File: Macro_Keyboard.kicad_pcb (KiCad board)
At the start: 6 copper layers, 109.7 x 84.3 mm, 106 parts, among them J1 USB_C_Receptacle_USB2.0, J2 USB_A, J3 USB_A, J4 USB_A, SW1 SW_Push, SW10 SW_DIP_x01, SW2 SW_DIP_x01, SW3 SW_DIP_x01, SW4 SW_DIP_x01, SW5 SW_DIP_x01, SW6 SW_DIP_x01, SW7 SW_DIP_x01, SW8 SW_DIP_x01, SW9 SW_DIP_x01, U1 STM32L432KCUx, U2 LD39050PU33R, U5 SRV05-4, U6 SRV05-4, Y1 12MHz

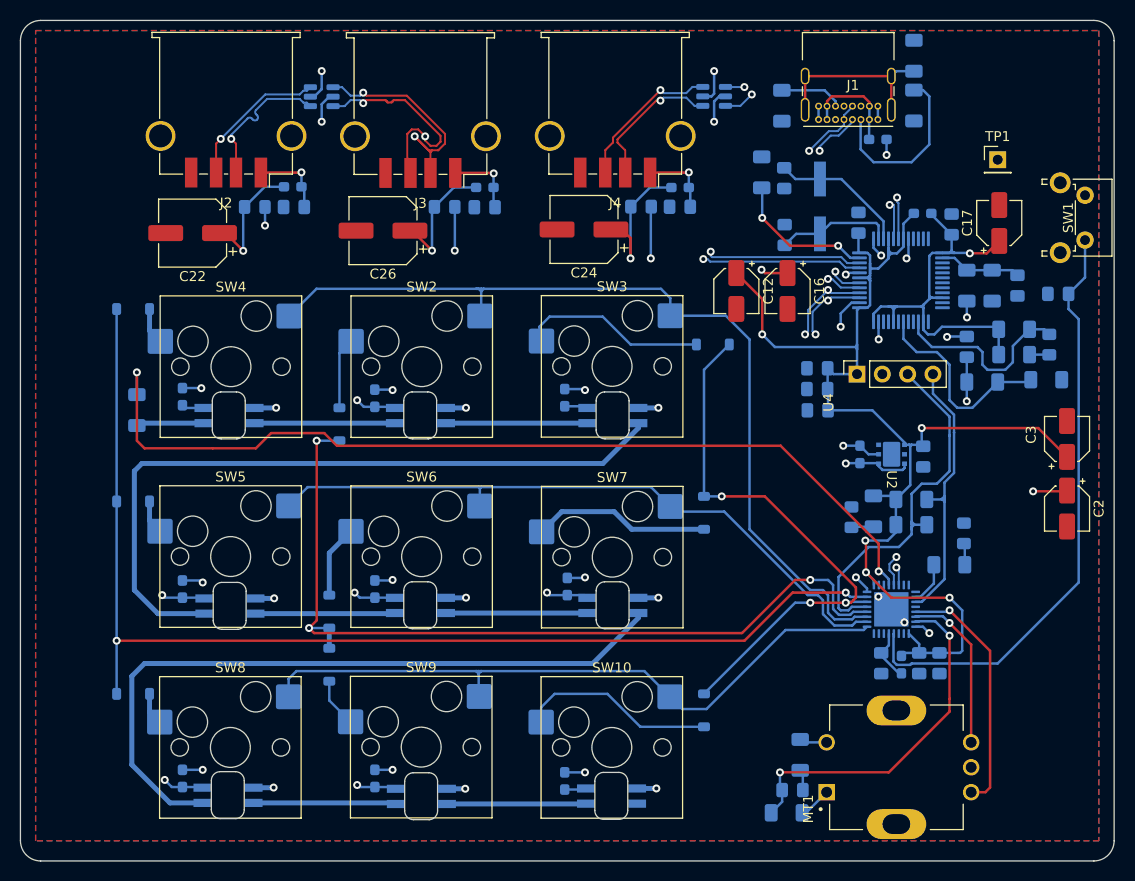
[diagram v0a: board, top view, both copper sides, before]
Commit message: Add files via upload
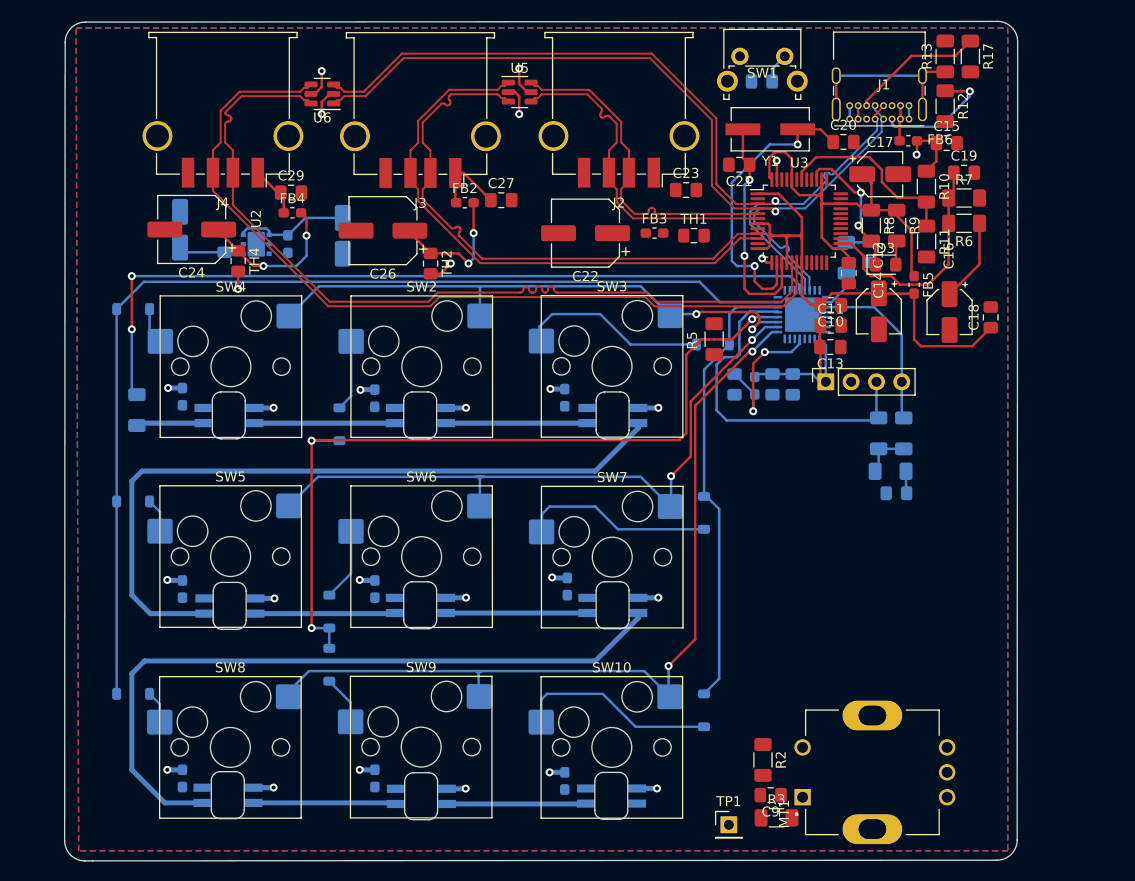
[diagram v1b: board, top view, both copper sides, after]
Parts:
- C10, C11, C13, C14, C15, C18, C19, C20, C21, C23, C27, C29, C9, D3, FB2, FB3, FB4, FB5, FB6, R10, R11, R12, R13, R17, R2, R3, R5, R6, R7, R8, R9, TH1, TH2, TH4, U3, U5, U6, Y1: moved to F.Cu
- C2, C3: moved to B.Cu
- moved C3 91.4 mm to (72.9, 60.6)
- moved C2 77.6 mm to (89.2, 61.2)
- moved C4 73.3 mm to (77.4, 61.8), turned to 90 degrees
- moved TP1 72.0 mm to (128.0, 120.3)
- moved U2 67.1 mm to (80.6, 62.1), turned to -90 degrees
- moved C1 61.1 mm to (83.7, 62.1), turned to -90 degrees
- moved TH1 44.2 mm to (124.5, 61.2)
- moved TH4 40.8 mm to (78.7, 63.8), turned to -90 degrees
- moved J2 39.4 mm to (116.9, 48.5)
- moved C22 39.4 mm to (113.6, 61.0)
- moved C23 39.4 mm to (123.7, 56.6), turned to 0 degrees
- moved C24 39.4 mm to (74.1, 60.6)
- moved J4 39.4 mm to (77.2, 48.5)
- moved U6 39.3 mm to (87.2, 47.0)
- moved C29 39.0 mm to (84.1, 56.9), turned to 0 degrees
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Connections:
- U5 pad 1: /USB/D_N2 -> /USB/D_P2
- U5 pad 3: /USB/D_P2 -> /USB/D_N2
- U5 pad 4: /USB/D_N1 -> /USB/D_P1
- U5 pad 6: /USB/D_P1 -> /USB/D_N1
- U6 pad 1: USBD_N -> USBD_P
- U6 pad 3: USBD_P -> USBD_N
- U6 pad 4: /USB/D_N3 -> /USB/D_P3
- U6 pad 6: /USB/D_P3 -> /USB/D_N3
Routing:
- net /USB/D_P1: track 96.7 -> 34.2 mm, vias 2 -> 0
- net /USB/D_N1: track 96.6 -> 34.2 mm, vias 2 -> 0
- net Net-(U1-NRST): track 60.4 -> 3.04 mm
- net GND: track 62.0 -> 9.63 mm, vias 18 -> 3
- net +3.3V: track 128.6 -> 84.1 mm, vias 5 -> 0
- net /USB/D_N3: track 46.7 -> 86.0 mm, vias 2 -> 0
- net /USB/D_P3: track 47.6 -> 86.2 mm, vias 2 -> 0
- net Net-(U1-PH3): track 35.8 -> 0.00 mm, vias 2 -> 0
- net ROW 0: track 89.9 -> 57.7 mm, vias 0 -> 2
- net Rotary_A: track 25.0 -> 0.00 mm, vias 1 -> 0
- net /USB/D_N2: track 77.7 -> 56.9 mm, vias 3 -> 0
- net /USB/D_P2: track 77.1 -> 57.0 mm, vias 3 -> 0
- net /USB/X1: track 11.8 -> 30.6 mm, vias 0 -> 2
- net ROW 2: track 68.5 -> 85.7 mm, vias 0 -> 2
- net Rotary_B: track 16.6 -> 0.00 mm, vias 1 -> 0
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- removed copper zone on In4.Cu, net GND
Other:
- board size 109.7 x 84.3 mm -> 95.6 x 84.2 mm
- copper layers 6 -> 4
